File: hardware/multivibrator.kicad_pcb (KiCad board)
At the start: 2 copper layers, 28 x 36 mm, 13 parts, among them J1 KLS2-EDR-5.08-02P-4, Q1 BC817, Q2 BC817

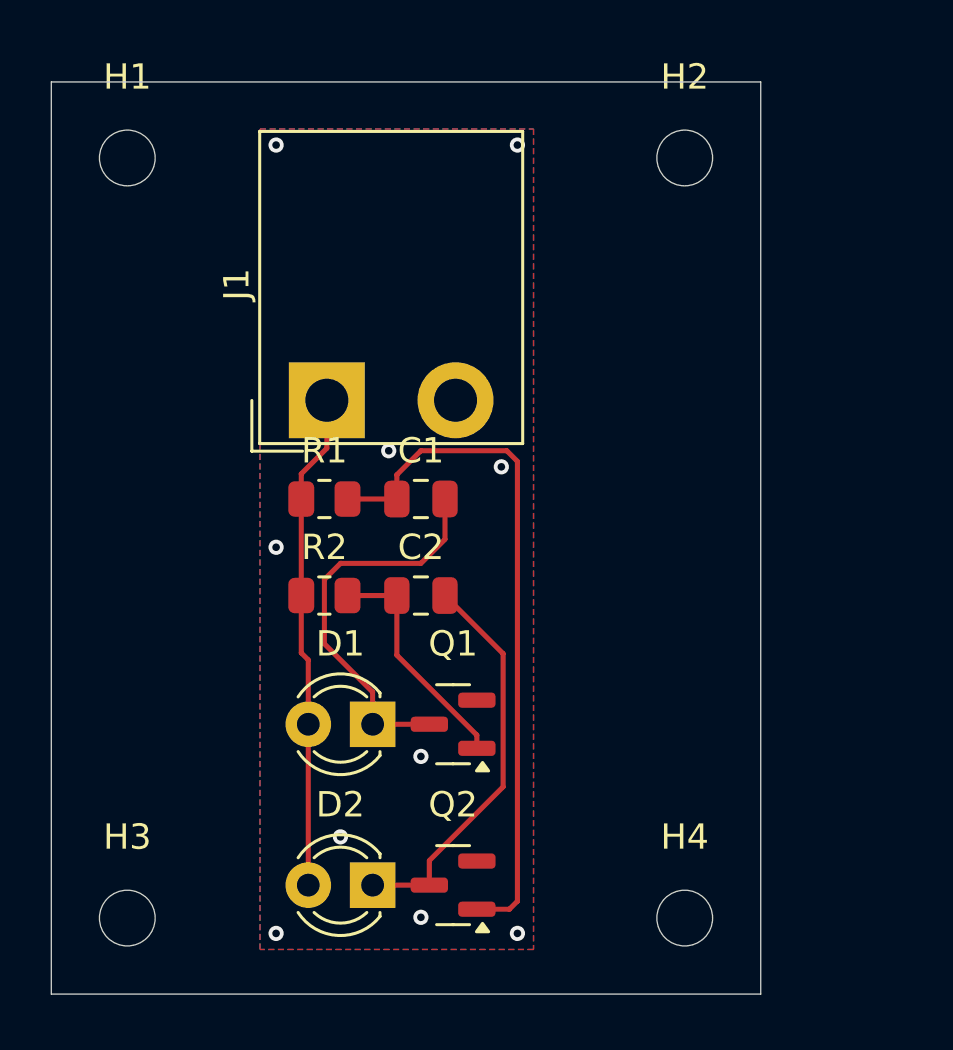
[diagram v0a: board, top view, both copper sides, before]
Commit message: учтены замечания
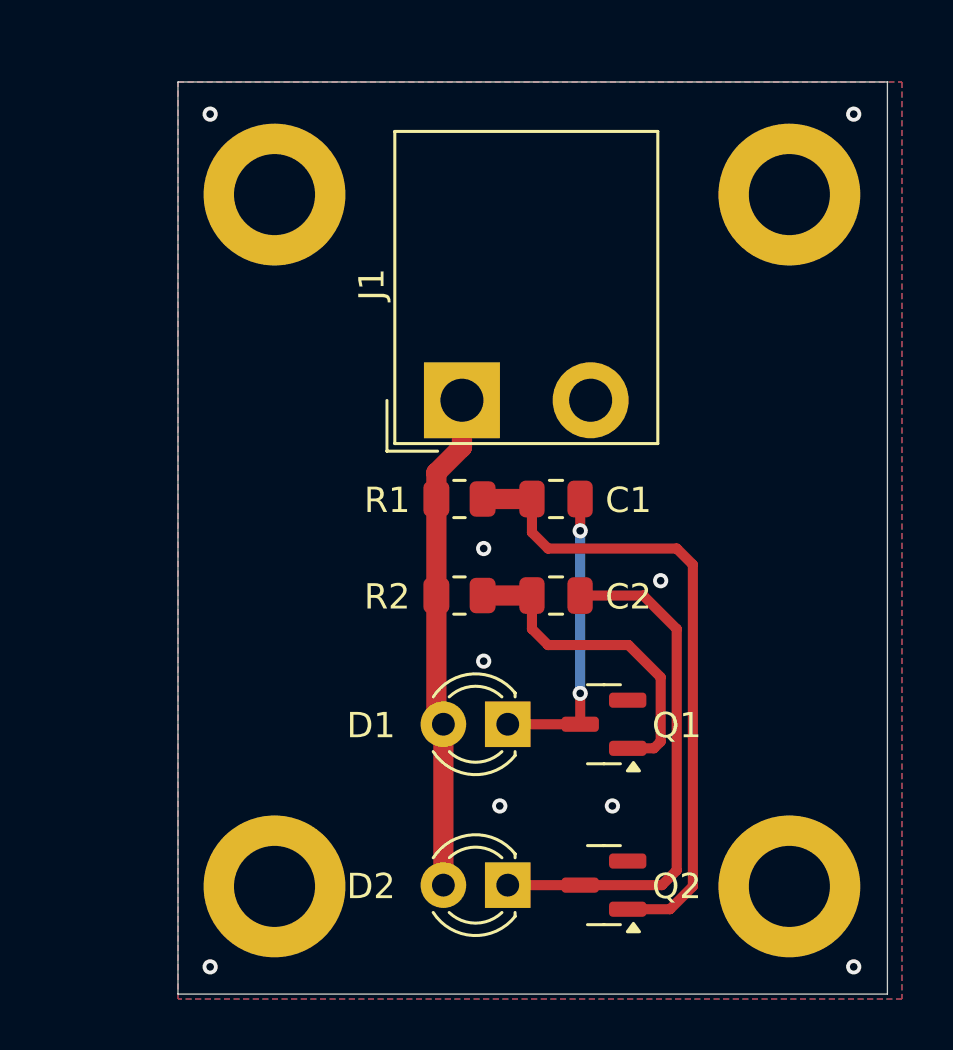
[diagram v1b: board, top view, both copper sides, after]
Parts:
- H1, H2, H3, H4: value MountingHole -> MountingHole_Pad; footprint MountingHole:MountingHole_2.2mm_M2 -> MountingHole:MountingHole_3.2mm_M3_DIN965_Pad
- moved H1 5.99 mm to (33.8, 34.4)
- moved Q1 5.95 mm to (46.8, 55.4)
- moved Q2 5.95 mm to (46.8, 61.7)
- moved H3 5.94 mm to (33.8, 61.8)
- moved C1 5.33 mm to (44.9, 46.5)
- moved C2 5.33 mm to (44.9, 50.3)
- moved D1 5.33 mm to (43.0, 55.4)
- moved D2 5.33 mm to (43.0, 61.7)
- moved J1 5.33 mm to (41.2, 42.6)
- moved R1 5.33 mm to (41.1, 46.5)
- moved R2 5.33 mm to (41.1, 50.3)
- moved H2 4.38 mm to (54.1, 34.4)
- moved H4 4.32 mm to (54.1, 61.8)
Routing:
- net Net-(D1-K): track 15.7 -> 11.1 mm, vias 0 -> 2
- net Net-(D2-K): track 15.8 -> 20.2 mm
- net Net-(Q1-B): track 9.29 -> 13.1 mm
- net Net-(Q2-B): track 28.0 -> 26.1 mm
- net +5V: track 19.7 -> 21.1 mm
- net GND: vias 10 -> 9
